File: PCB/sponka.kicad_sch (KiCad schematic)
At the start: 3 parts, among them J1 Conn_01x03_Pin, U1 CH32V003FxUx

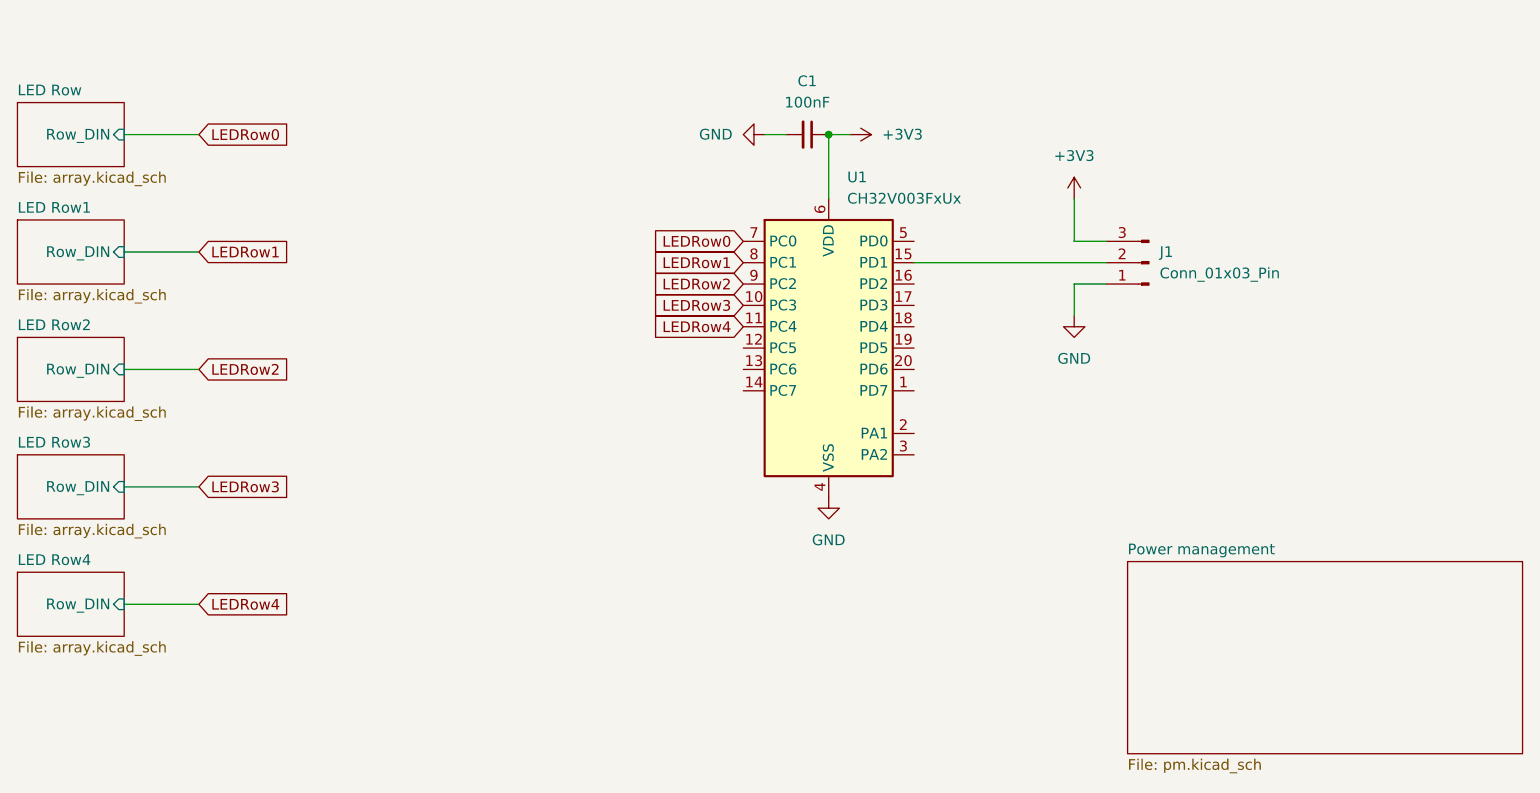
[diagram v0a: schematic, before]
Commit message: Made first PCB
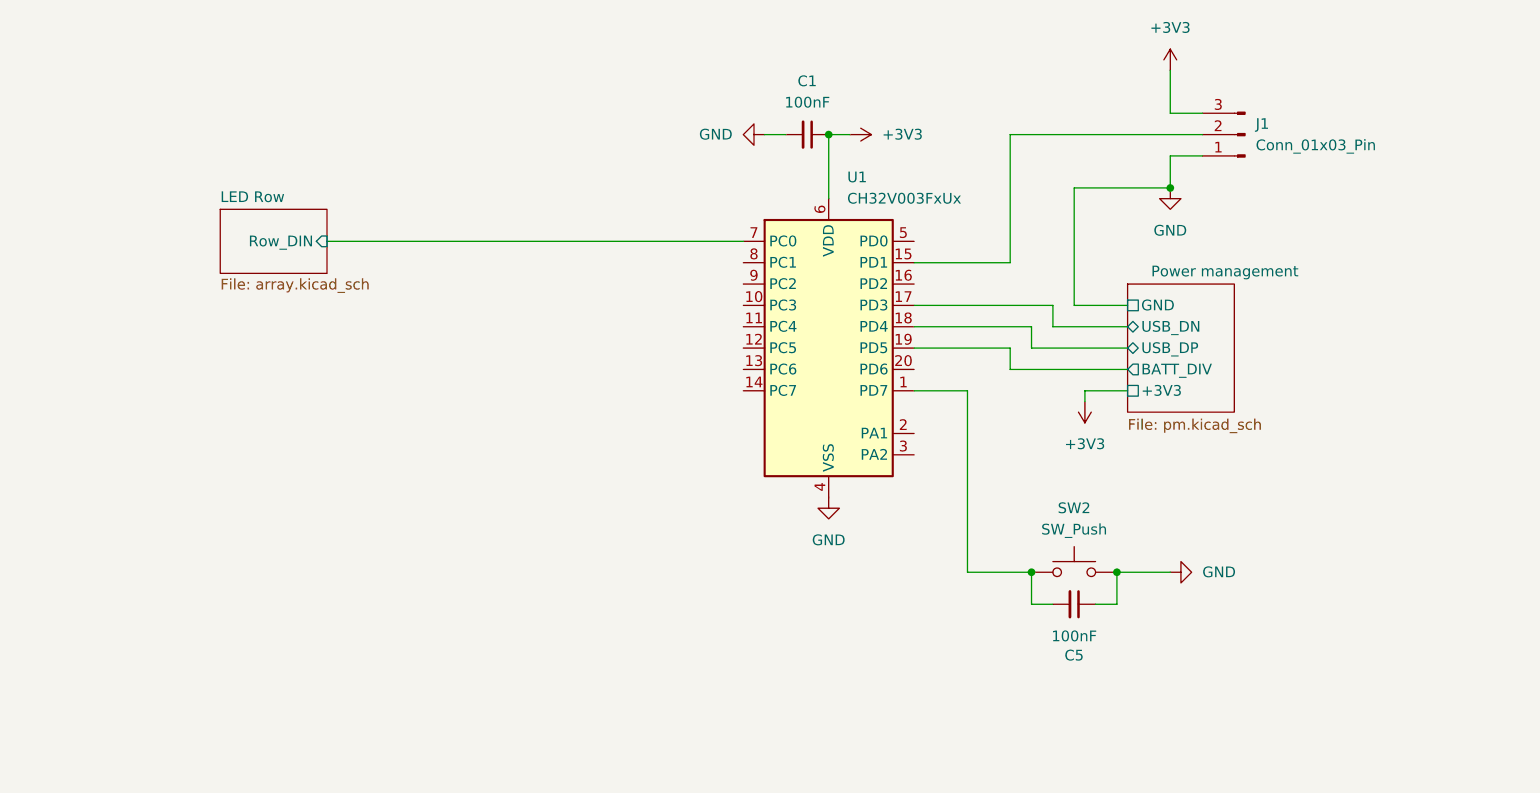
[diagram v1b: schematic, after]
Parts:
- added C5: 100nF, Capacitor_SMD:C_0402_1005Metric, symbol Device:C_Small
- added SW2: SW_Push, Button_Switch_SMD:SW_SPST_B3U-1000P-B, symbol Switch:SW_Push
- C1: footprint Capacitor_SMD:C_0504_1310Metric -> Capacitor_SMD:C_0402_1005Metric
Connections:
- net GND: now also C5.1, SW2.2
- net at U1.1 (PD7): now also C5.2, SW2.1
- net Power management/USB_DN: now reaches U1.17 (PD3)
- net Power management/USB_DP: now reaches U1.18 (PD4)
- net Power management/BATT_DIV: now reaches U1.19 (PD5)
- net LEDRow0 renamed LED Row/Row_DIN
- net LEDRow1: no longer names the net of U1.8 (PC1)
- net LEDRow2: no longer names the net of U1.9 (PC2)
- net LEDRow3: no longer names the net of U1.10 (PC3)
- net LEDRow4: no longer names the net of U1.11 (PC4)
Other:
- removed sheet LED Row1
- removed sheet LED Row2
- removed sheet LED Row3
- removed sheet LED Row4
- sheet Power management ports: added +3V3, BATT_DIV, GND, USB_DN, USB_DP; removed none
- moved on the sheet: J1
